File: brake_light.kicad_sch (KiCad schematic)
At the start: 12 parts, among them Q1 AO3401A, Q2 AO3401A, U1 US2881LUA-AAA-000-BU, U2 US2881LUA-AAA-000-BU

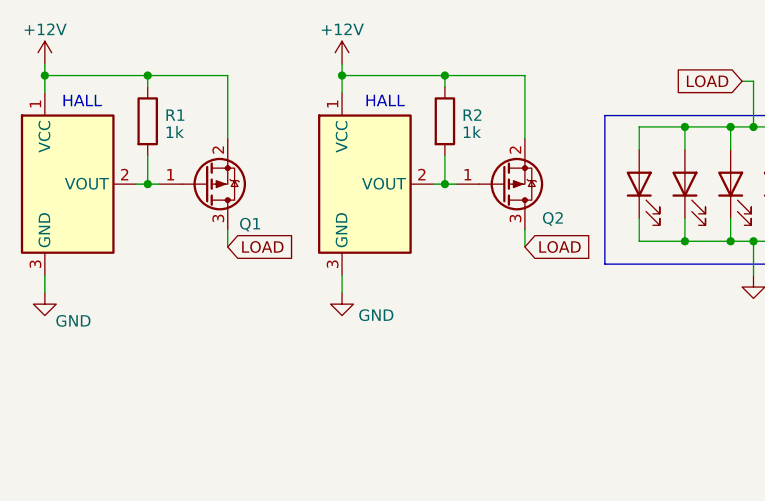
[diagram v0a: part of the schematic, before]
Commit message: handled layout
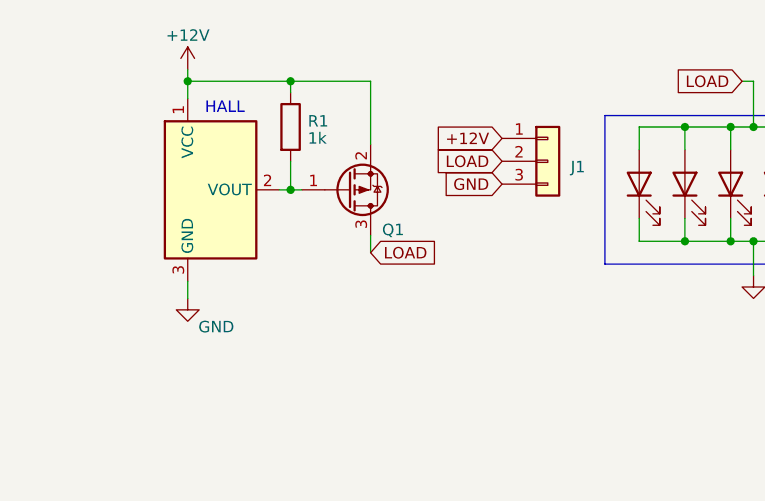
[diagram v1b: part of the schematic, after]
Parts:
- removed Q2: AO3401A, Package_TO_SOT_SMD:SOT-23, symbol Transistor_FET:AO3401A
- removed R2: 1k, symbol Device:R
- removed U2: US2881LUA-AAA-000-BU, Package_TO_SOT_SMD:SOT-23W, symbol Sensor_Magnetic:A1101ELHL
- added J1: Conn_01x03, connector:3_smd_tab, symbol Connector_Generic:Conn_01x03
- R1: footprint (none) -> Resistor_SMD:R_0805_2012Metric
- U1: value US2881LUA-AAA-000-BU -> TMAG5115
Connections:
- net +12V: now also J1.1 (Pin_1)
- net GND: now also J1.3 (Pin_3)
- net LOAD: now also J1.2 (Pin_2)
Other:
- moved on the sheet: Q1, R1
